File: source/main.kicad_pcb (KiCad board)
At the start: 2 copper layers, 85.6 x 54 mm, 61 parts, among them P1 USB_Type_C_Receptacle_16_pin

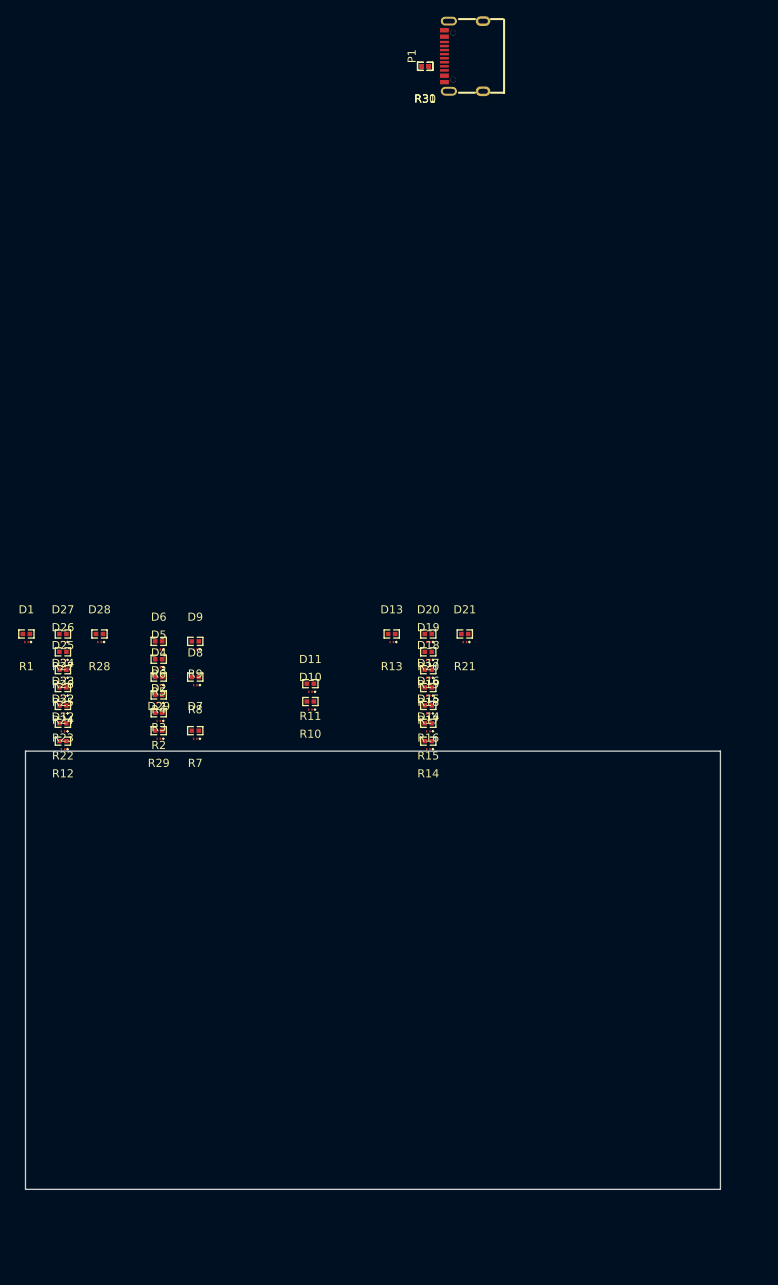
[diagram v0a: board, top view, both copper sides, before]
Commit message: Fix layout
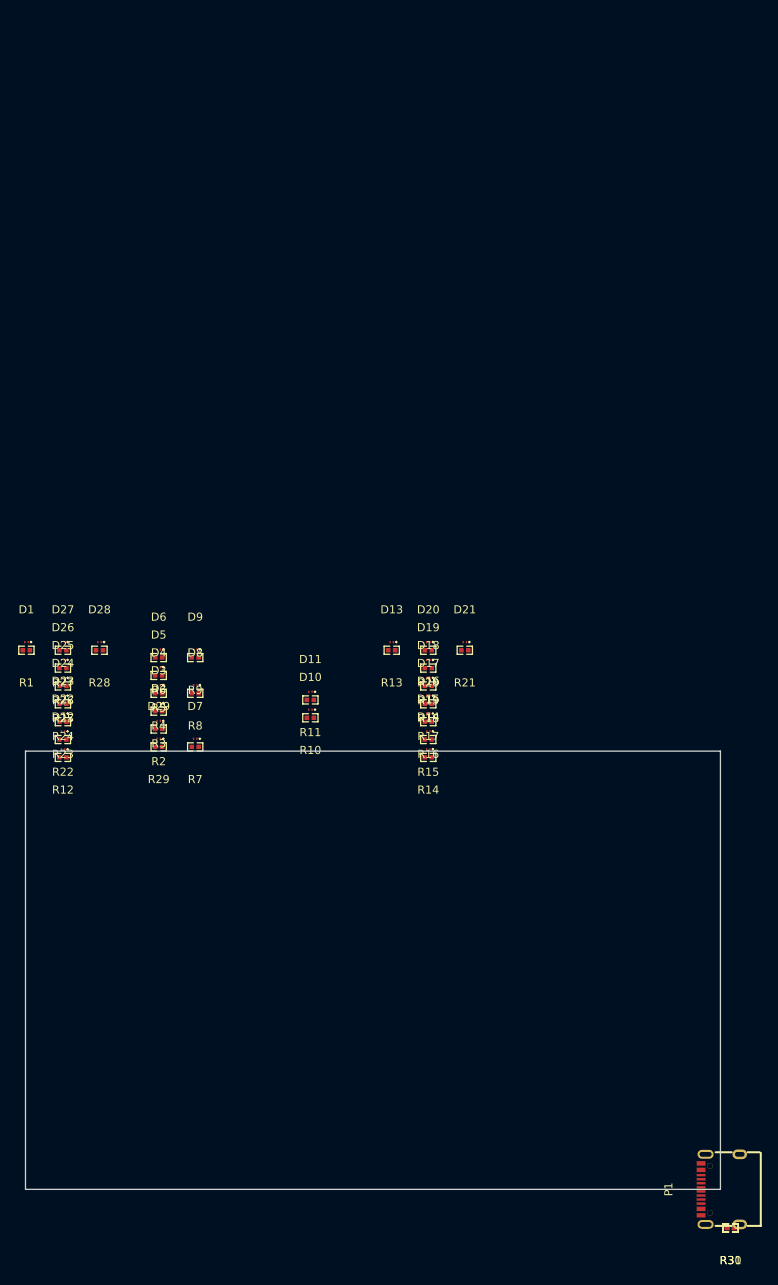
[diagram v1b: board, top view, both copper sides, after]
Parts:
- moved R30 147.9 mm to (86.8, 58.7)
- moved R31 147.9 mm to (86.8, 58.7)
- moved P1 143.1 mm to (85.6, 54.0)
- moved R19 2.00 mm to (49.6, -10.2)
- moved R26 2.00 mm to (4.61, -10.2)
- moved R12 2.00 mm to (4.61, 0.77)
- moved R14 2.00 mm to (49.6, 0.77)
- moved R15 2.00 mm to (49.6, -1.43)
- moved R22 2.00 mm to (4.61, -1.43)
- moved R1 2.00 mm to (0.11, -12.4)
- moved R13 2.00 mm to (45.1, -12.4)
- moved R16 2.00 mm to (49.6, -3.63)
- moved R17 2.00 mm to (49.6, -5.83)
- moved R18 2.00 mm to (49.6, -8.03)
- moved R20 2.00 mm to (49.6, -12.4)
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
